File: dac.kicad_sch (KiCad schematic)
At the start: 15 parts, among them U15 74LV32, U17 74LV32, U30 74LV08, U31 74LV08

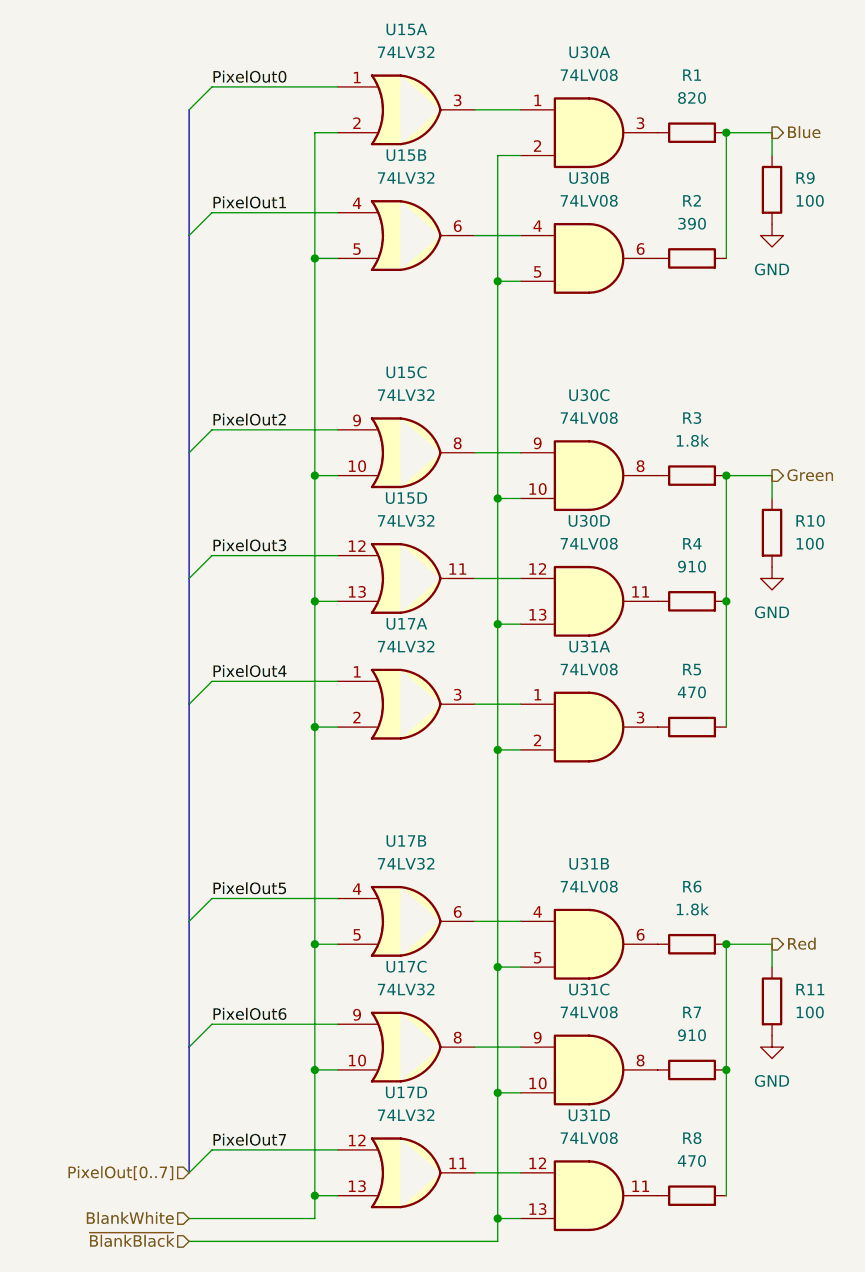
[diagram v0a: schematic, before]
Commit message: Work on layout/routing
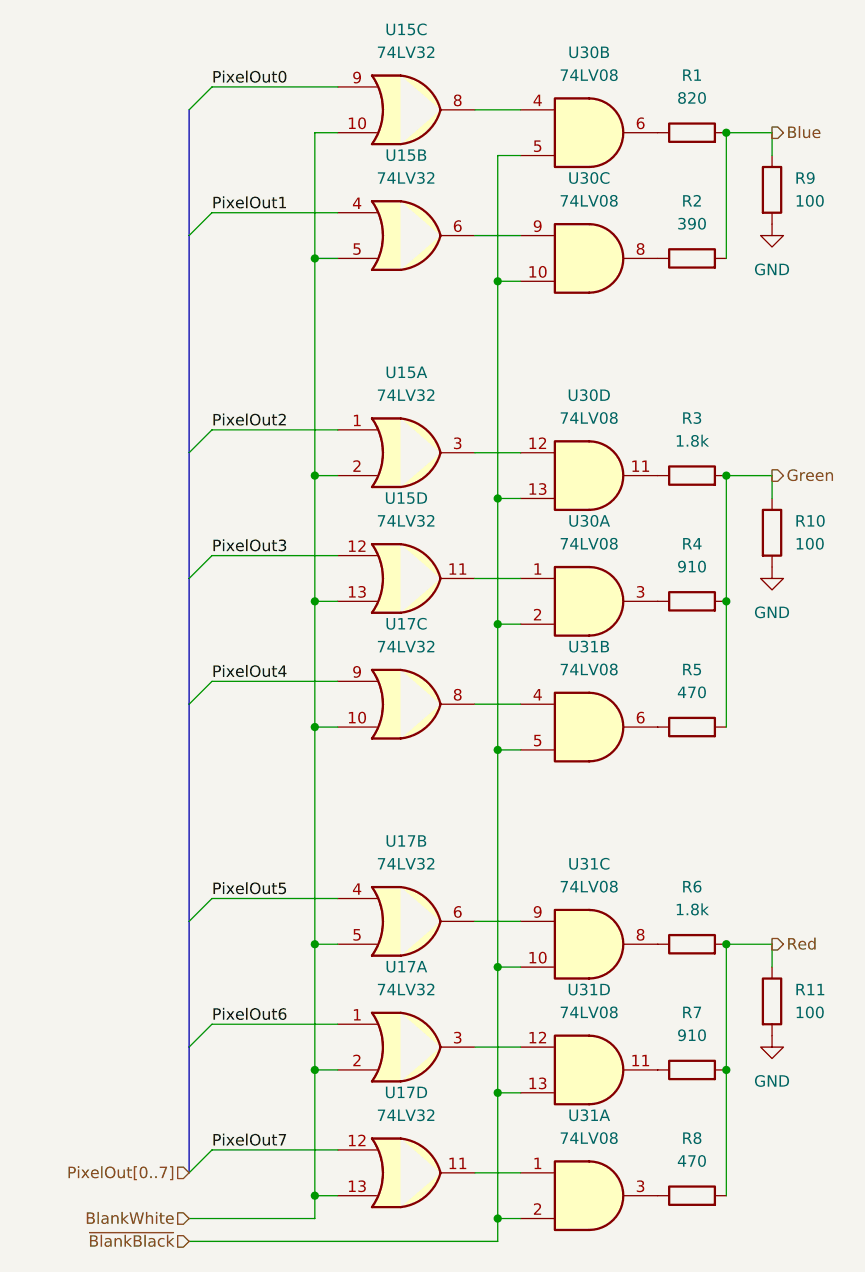
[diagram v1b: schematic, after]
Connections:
- net PixelOut0: now also U15.9; no longer U15.1
- net PixelOut2: now also U15.1; no longer U15.9
- net PixelOut4: now also U17.9; no longer U17.1
- net PixelOut6: now also U17.1; no longer U17.9
- net at U17.6: now also U31.9; no longer U31.4
- net at U30.4: now also U15.8; no longer U15.6
- net at U30.6: now also R1.1; no longer R2.1
- net at U15.11: now also U30.1; no longer U30.12
- net at U30.9: now also U15.6; no longer U15.8
- net at U30.8: now also R2.1; no longer R3.1
- net at U30.11: now also R3.1; no longer R4.1
- net at U17.11: now also U31.1; no longer U31.12
- net at R5.1: now also U31.6; no longer U31.3
- net at R6.1: now also U31.8; no longer U31.6
- net at U17.8: now also U31.4; no longer U31.9
- net at U17.3: now also U31.12; no longer U31.1
- net at U30.3: now also R4.1; no longer R1.1
- net at R8.1: now also U31.3; no longer U31.11
- net at R7.1: now also U31.11; no longer U31.8
- net at U15.3: now also U30.12; no longer U30.1
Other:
- moved on the sheet: U15A, U15C, U17A, U17C, U30A, U30B, U30C, U30D, U31A, U31B, U31C, U31D
